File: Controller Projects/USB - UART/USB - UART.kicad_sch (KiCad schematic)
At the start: 9 parts, among them J1 USB_C_Receptacle_USB2.0_14P, J2 Conn_01x04, U1 CH340C

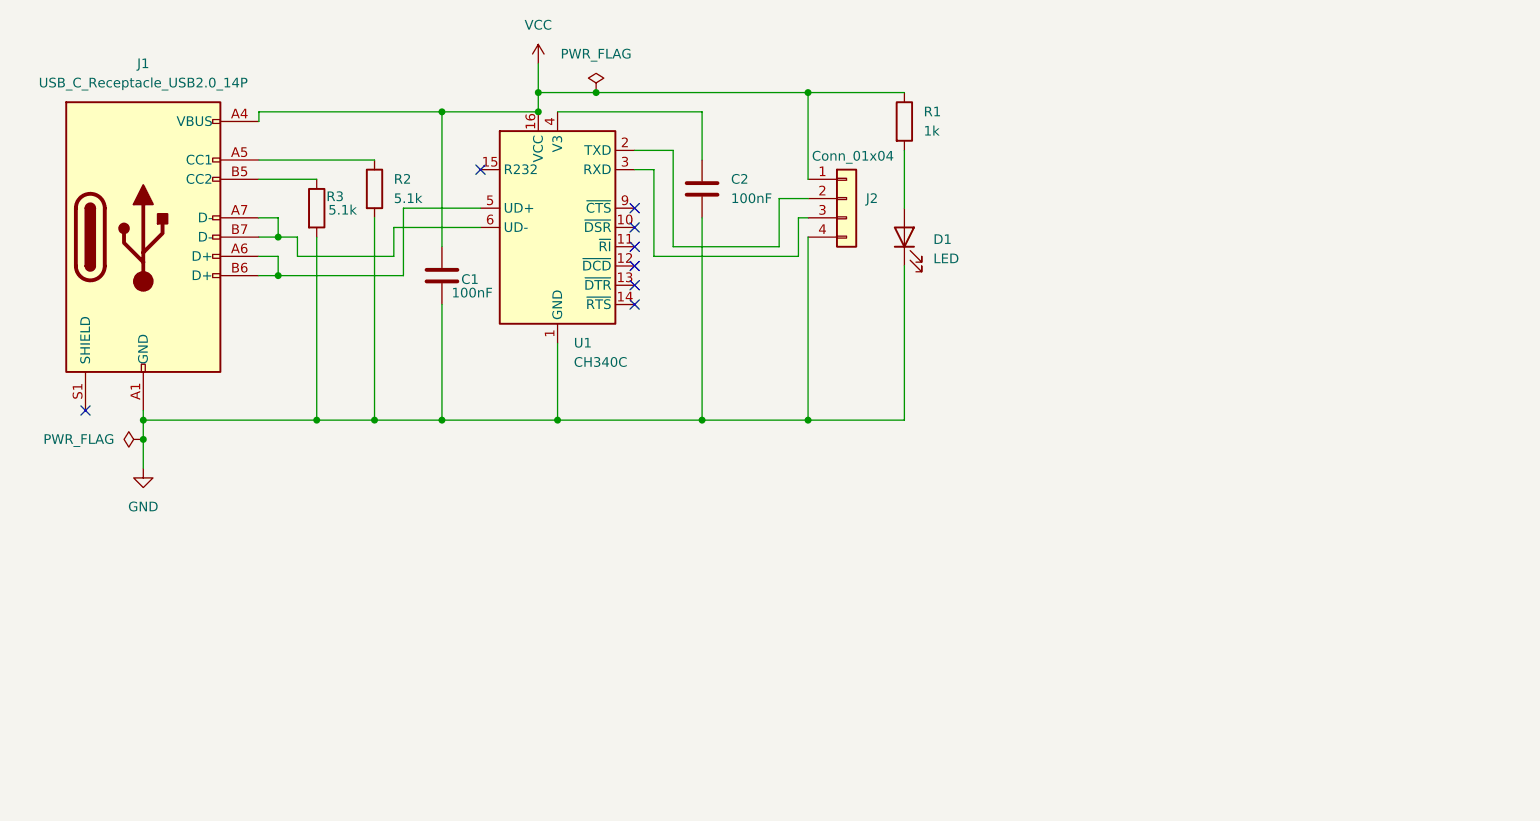
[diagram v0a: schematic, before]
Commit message: Initial Commit
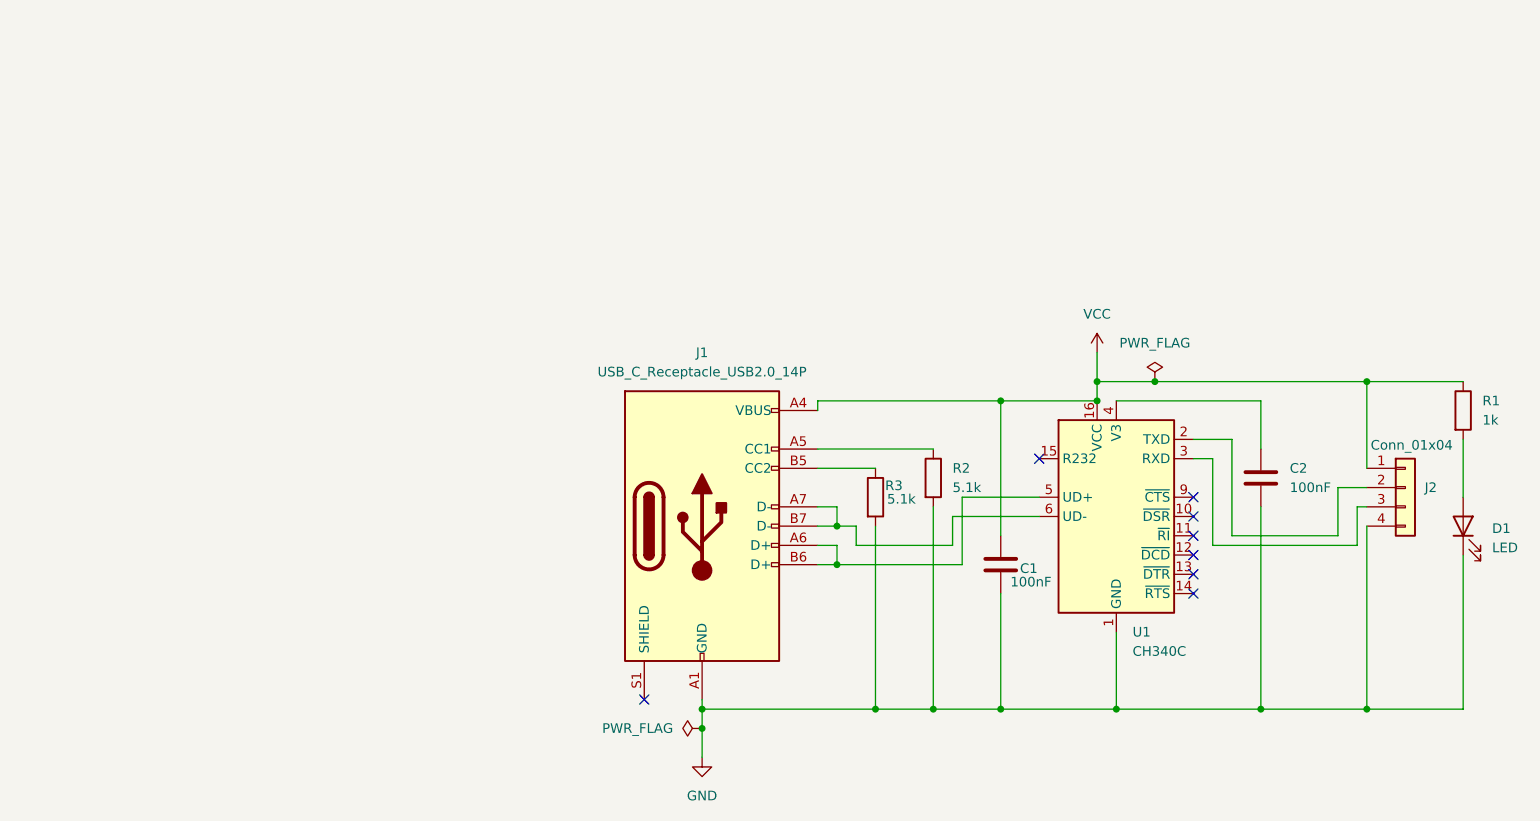
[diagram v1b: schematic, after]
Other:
- moved on the sheet: C1, C2, D1, J1, J2, R1, R2, R3, U1
